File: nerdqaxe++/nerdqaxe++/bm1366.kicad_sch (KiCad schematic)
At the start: 82 parts, among them J2 Conn_01x06, U19 BM1370_mode1, U20 BM1370_mode1, U25 BM1370_mode1, U26 BM1370_mode1, U35 TXU0304PW, U8 25MHz

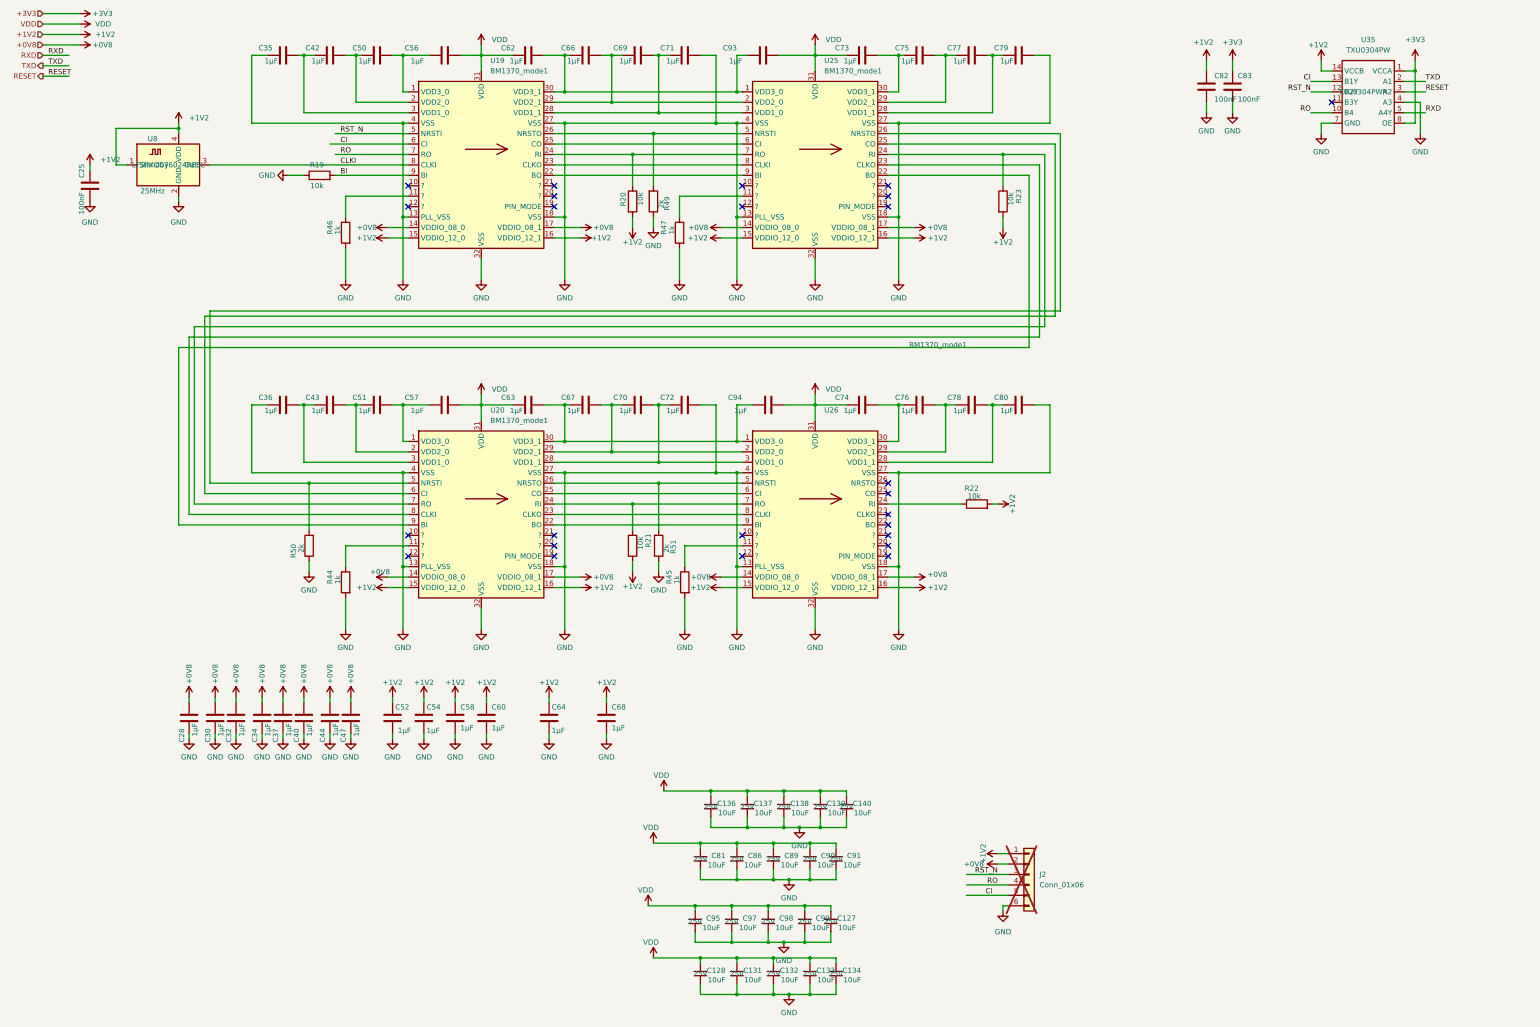
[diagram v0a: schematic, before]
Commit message: 5v
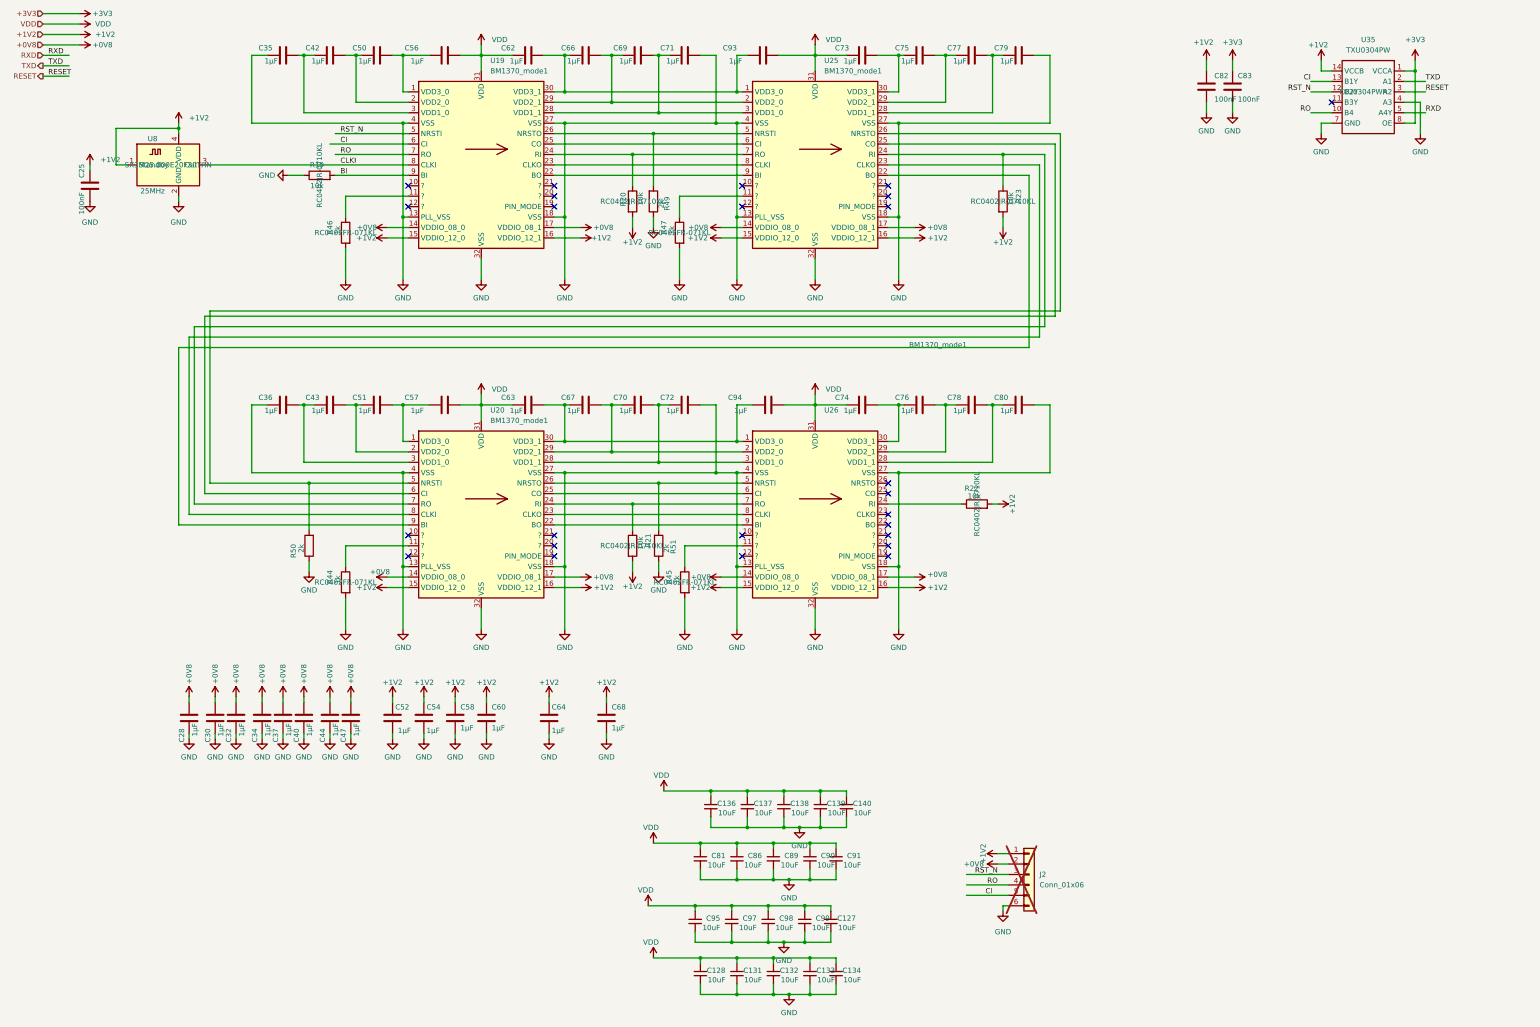
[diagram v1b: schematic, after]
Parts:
- C127, C128, C131, C132, C133, C134, C136, C137, C138, C139, C140, C81, C86, C89, C90, C91, C95, C97, C98, C99: DK 490-18214-1-ND -> (none); Voltage 25V -> (none)
- C25, C82, C83: PARTNO (none) -> CL05A104KO5NNNC
- C28, C30, C32, C34, C35, C36, C37, C40, C42, C43, C44, C47, C50, C51, C52, C54, C56, C57, C58, C60, C62, C63, C64, C66, C67, C68, C69, C70, C71, C72, C73, C74, C75, C76, C77, C78, C79, C80, C93, C94: PARTNO (none) -> EMK105BJ105MV-F
- R19, R20, R21, R22, R23: PARTNO (none) -> RC0402JR-0710KL
- R44, R45, R46, R47: PARTNO (none) -> RC0402FR-071KL
- U8: PARTNO LFSPXO076024REEL -> SX3M25.000E20F30THN

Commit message: finishing up
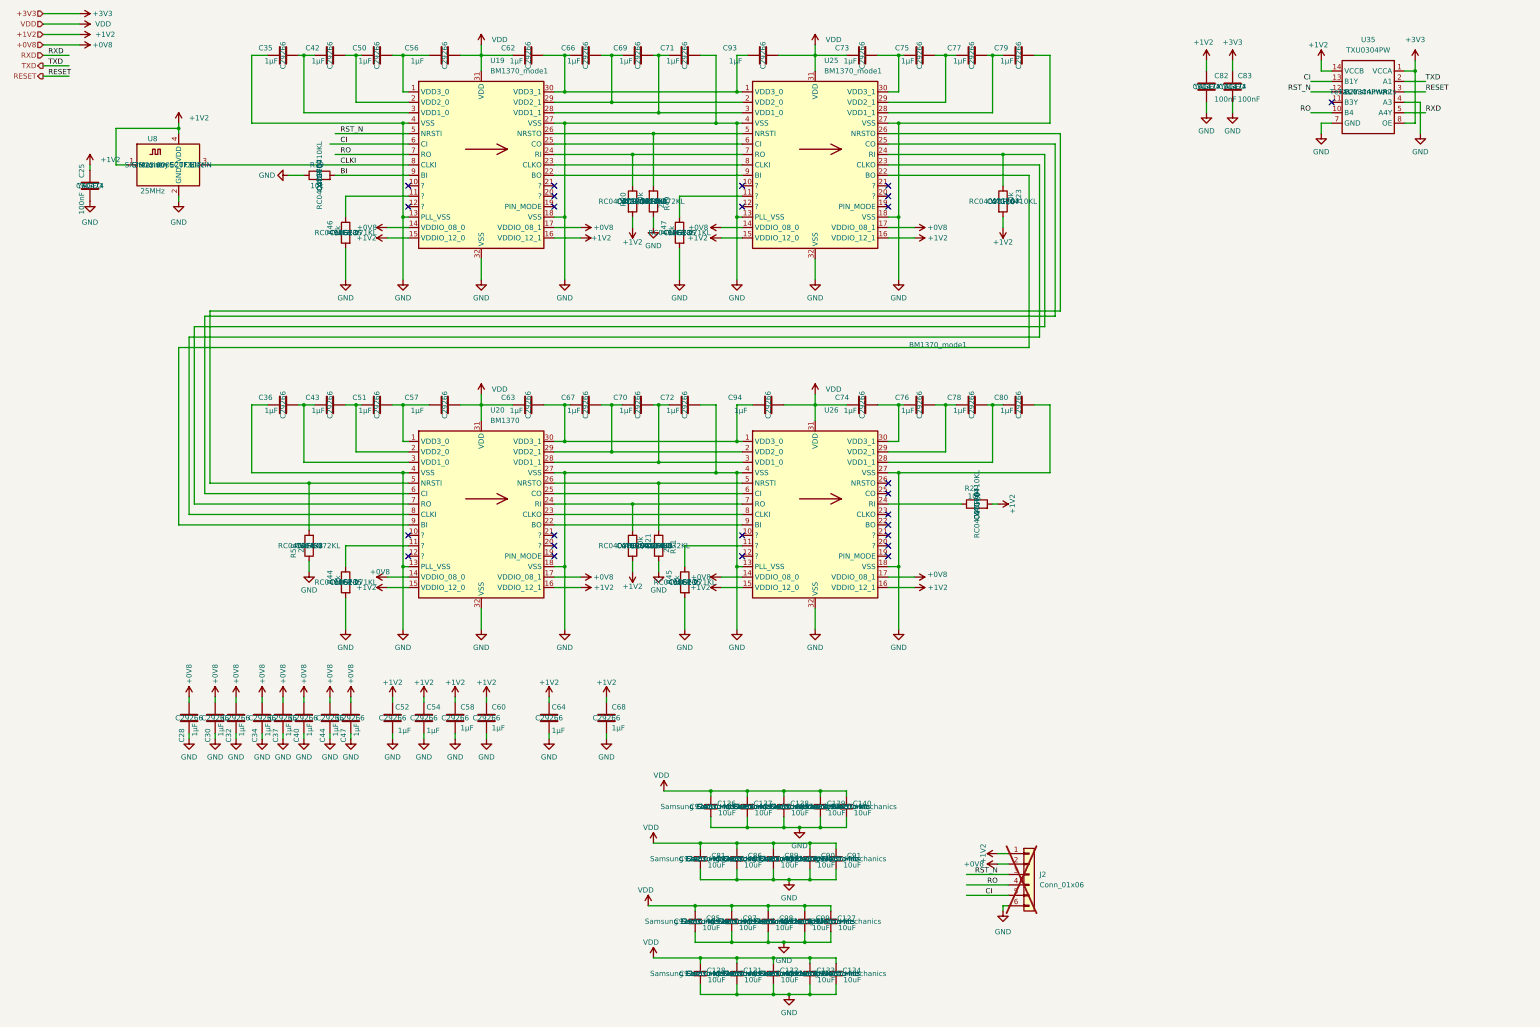
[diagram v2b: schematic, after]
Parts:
- C127, C128, C131, C132, C133, C134, C136, C137, C138, C139, C140, C81, C86, C89, C90, C91, C95, C97, C98, C99: LCSC (none) -> C92487 Hot; Manufacturer  (none) -> Samsung Electro-Mechanics; PARTNO GRM188R61E106KA73D -> CL10A106MO8NQNC
- C25, C82, C83: LCSC (none) -> C60474; Manufacturer  (none) -> YAGEO; PARTNO CL05A104KO5NNNC -> CC0402KRX7R7BB104
- C28, C30, C32, C34, C35, C36, C37, C40, C42, C43, C44, C47, C50, C51, C52, C54, C56, C57, C58, C60, C62, C63, C64, C66, C67, C68, C69, C70, C71, C72, C73, C74, C75, C76, C77, C78, C79, C80, C93, C94: LCSC (none) -> C29266; PARTNO EMK105BJ105MV-F -> CL05A105KO5NNNC
- R19, R20, R21, R22, R23: LCSC (none) -> C471764; Manufacturer  (none) -> YAGEO; PARTNO RC0402JR-0710KL -> RC0402DR-0710KL
- R44, R45, R46, R47: LCSC (none) -> C106235; Manufacturer  (none) -> YAGEO
- R49, R50, R51: LCSC (none) -> C60488; Manufacturer  (none) -> YAGEO; PARTNO (none) -> RC0402FR-072KL
- U19, U25, U26: footprint myfootprints:BM1370 -> qaxe:BM1370
- U20: value BM1370_mode1 -> BM1370; footprint myfootprints:BM1370 -> qaxe:BM1370
- U35: Manufacturer  (none) -> Texas Instruments
- U8: Manufacturer  (none) -> Shenzhen SCTF Elec

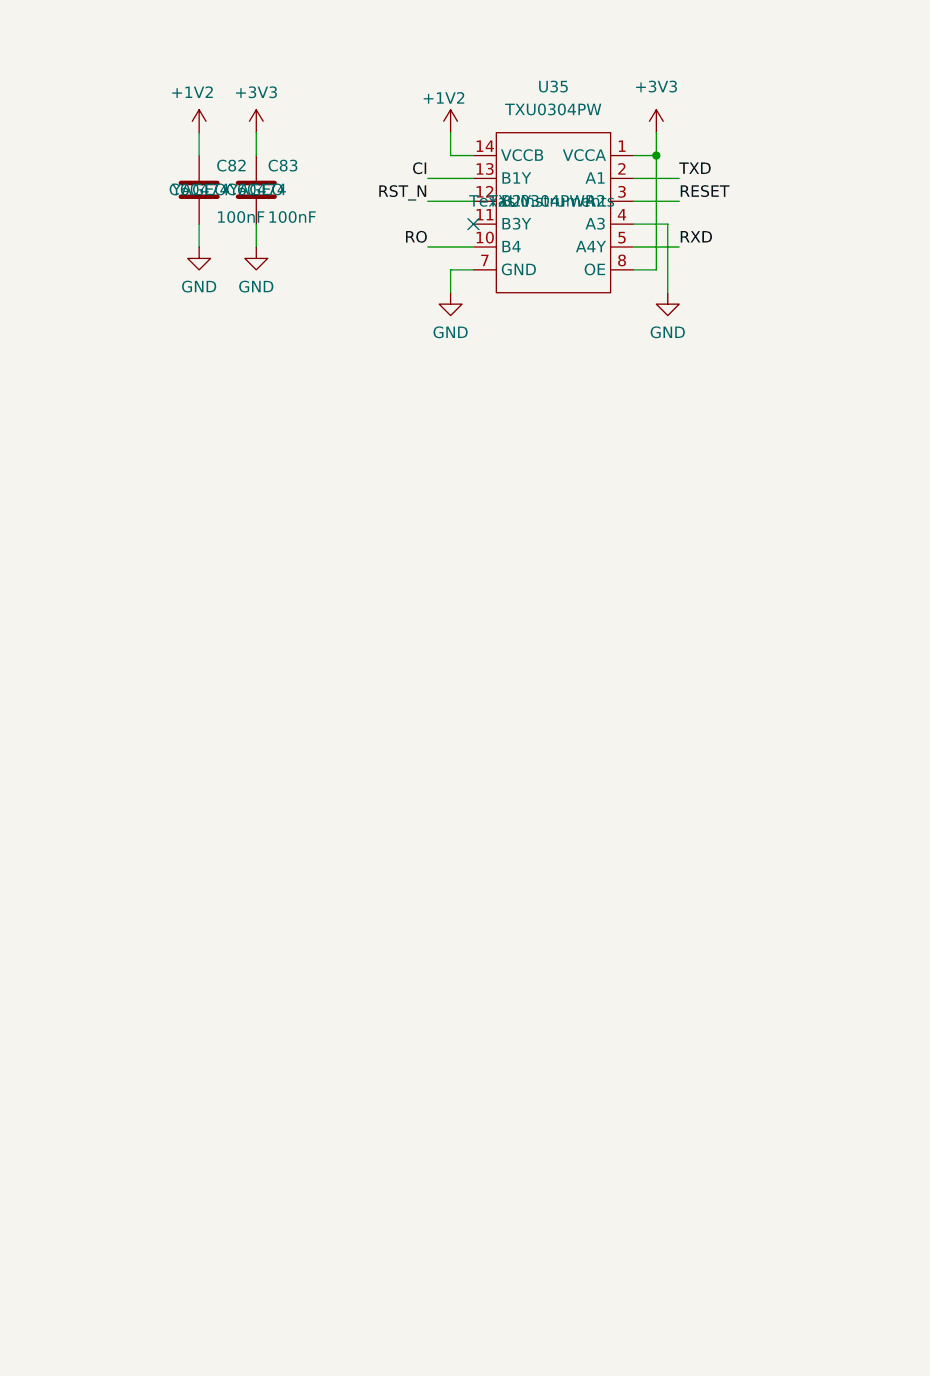
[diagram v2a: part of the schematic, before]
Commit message: level shifter
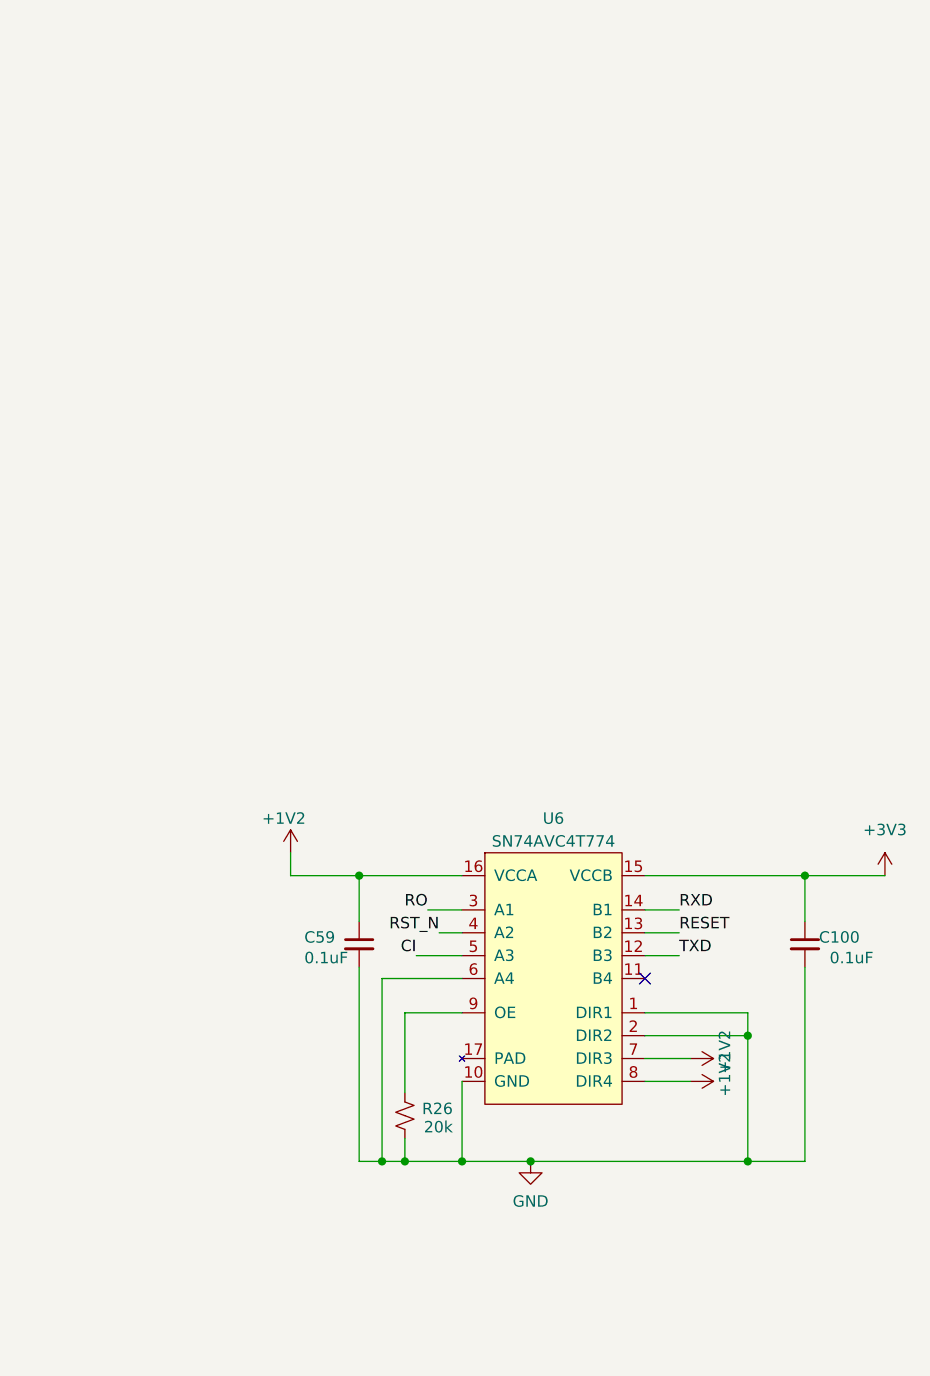
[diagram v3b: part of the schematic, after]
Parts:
- removed C82, C83: 100nF, Capacitor_SMD:C_0402_1005Metric, symbol Device:C
- removed U35: TXU0304PW, Package_SO:TSSOP-14_4.4x5mm_P0.65mm, symbol mylib7:TXU0304
- added C100, C59: 0.1uF, Capacitor_SMD:C_0402_1005Metric, symbol Device:C_Small
- added R26: 20k, Resistor_SMD:R_0402_1005Metric, symbol Device:R_Small_US
- added U6: SN74AVC4T774, qaxe:BQB0016A-MFG, symbol bitaxe:SN74AVC4T774-BQB
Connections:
- net +1V2: now also C59.1, U6.16 (VCCA), U6.7 (DIR3), U6.8 (DIR4)
- net +3V3: now also C100.1, U6.15 (VCCB)
- net CI: now also U6.5 (A3)
- net GND: now also C100.2, C59.2, R26.1, U6.1 (DIR1), U6.10 (GND), U6.2 (DIR2), U6.6 (A4)
- net RESET: now also U6.13 (B2)
- net RO: now also U6.3 (A1)
- net RST_N: now also U6.4 (A2)
- net RXD: now also U6.14 (B1)
- net TXD: now also U6.12 (B3)
- new net: R26.2, U6.9 (OE)
